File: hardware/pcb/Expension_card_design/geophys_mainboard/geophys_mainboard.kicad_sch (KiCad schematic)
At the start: 0 parts

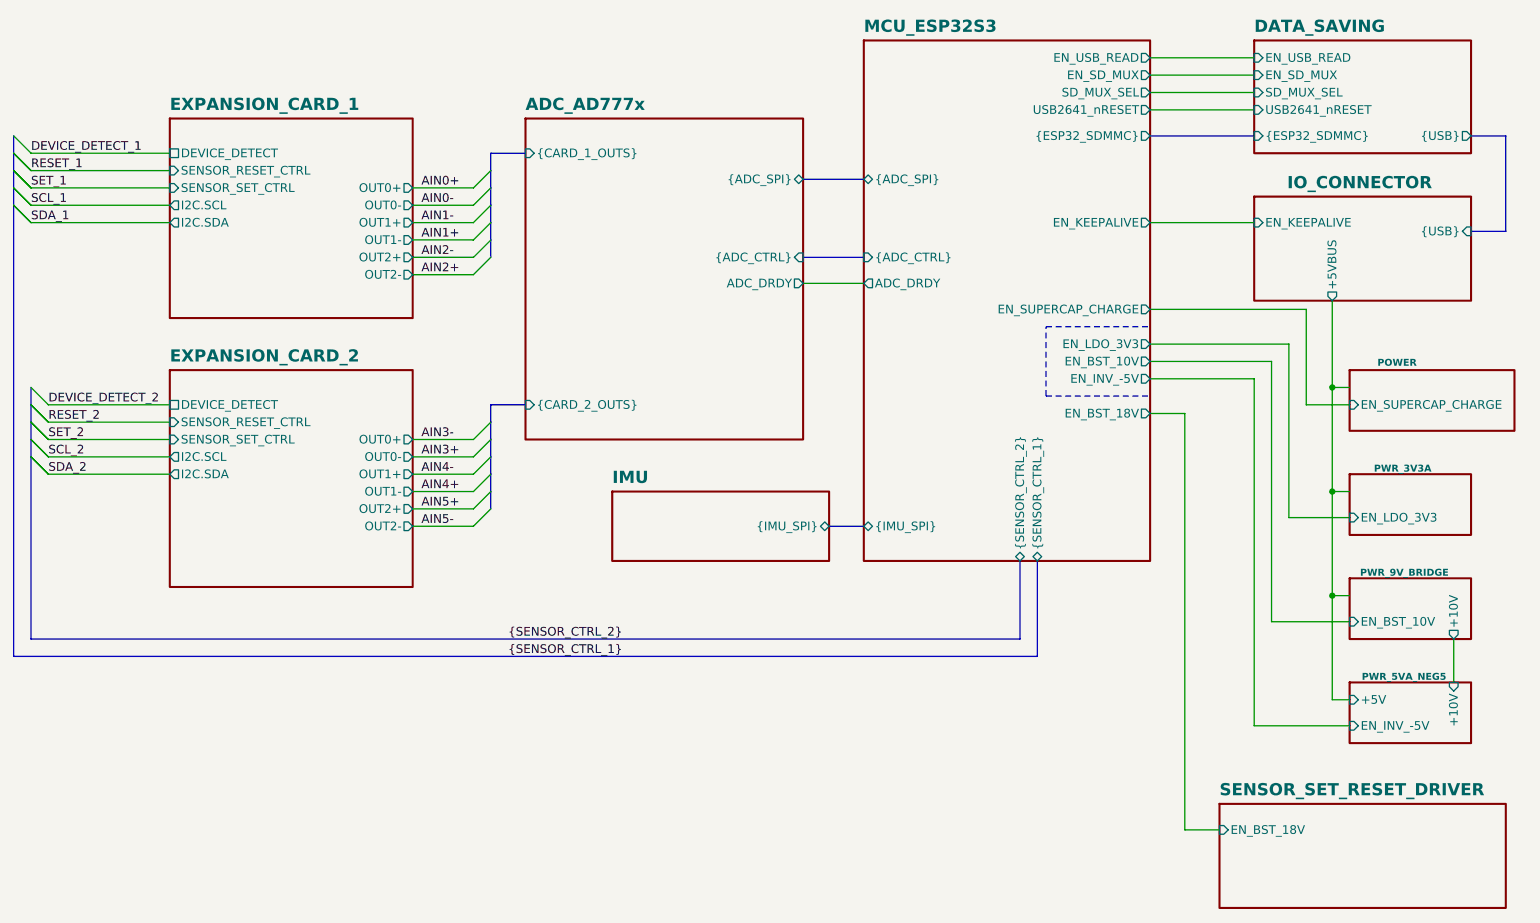
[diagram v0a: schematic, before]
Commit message: ...
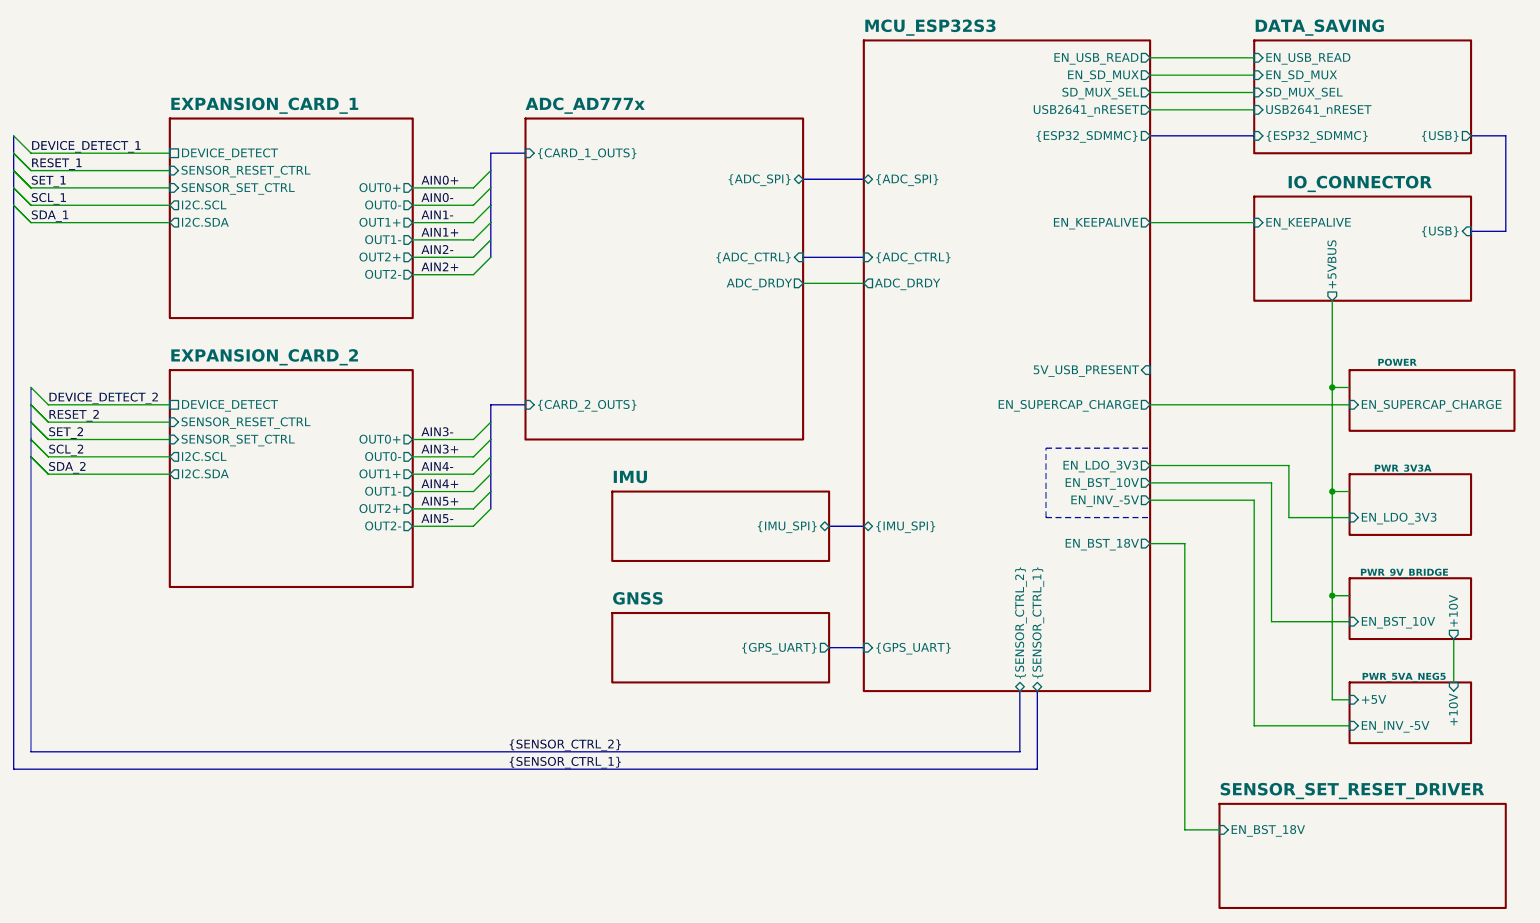
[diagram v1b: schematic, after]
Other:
- added sheet GNSS (schematics/GNSS.kicad_sch)
- sheet MCU_ESP32S3 ports: added 5V_USB_PRESENT, {GPS_UART}; removed none
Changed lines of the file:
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@@
-		)
-	)
-	(bus
-		(pts
-			(xy 176.53 102.87) (xy 176.53 114.3)
-		)
-		(stroke
-			(width 0)
-			(type default)
 		)
 	)
@@
 	(wire
 		(pts
-			(xy 195.58 73.66) (xy 213.36 73.66)
-		)
-		(stroke
-			(width 0)
-			(type default)
-		)
-	)
-	(bus
-		(pts
-			(xy 29.21 116.84) (xy 179.07 116.84)
+			(xy 195.58 91.44) (xy 213.36 91.44)
+		)
+		(stroke
+			(width 0)
+			(type default)
+		)
+	)
+	(bus
+		(pts
+			(xy 29.21 133.35) (xy 179.07 133.35)
 		)
 		(stroke
@@
 	(wire
 		(pts
-			(xy 218.44 80.01) (xy 218.44 66.04)
-		)
-		(stroke
-			(width 0)
-			(type default)
-		)
-	)
-	(wire
-		(pts
 			(xy 87.63 55.88) (xy 96.52 55.88)
 		)
@@
 	(bus
 		(pts
+			(xy 148.59 115.57) (xy 153.67 115.57)
+		)
+		(stroke
+			(width 0)
+			(type default)
+		)
+	)
+	(bus
+		(pts
 			(xy 29.21 48.26) (xy 29.21 50.8)
 		)
@@
 	(bus
 		(pts
+			(xy 176.53 121.92) (xy 176.53 130.81)
+		)
+		(stroke
+			(width 0)
+			(type default)
+		)
+	)
+	(bus
+		(pts
 			(xy 195.58 40.64) (xy 210.82 40.64)
 		)
@@
 	(bus
 		(pts
-			(xy 31.75 114.3) (xy 176.53 114.3)
+			(xy 31.75 130.81) (xy 176.53 130.81)
 		)
 		(stroke
@@
 	(polyline
 		(pts
-			(xy 180.34 78.74) (xy 195.58 78.74)
+			(xy 180.34 96.52) (xy 195.58 96.52)
 		)
 		(stroke
@@
 	(bus
 		(pts
-			(xy 31.75 87.63) (xy 31.75 114.3)
+			(xy 31.75 87.63) (xy 31.75 130.81)
 		)
 		(stroke
@@
 	(wire
 		(pts
-			(xy 210.82 76.2) (xy 210.82 127)
+			(xy 210.82 93.98) (xy 210.82 127)
 		)
 		(stroke
@@
 	(polyline
 		(pts
-			(xy 180.34 68.58) (xy 195.58 68.58)
+			(xy 180.34 86.36) (xy 195.58 86.36)
 		)
 		(stroke
@@
 		)
 	)
+	(bus
+		(pts
+			(xy 179.07 121.92) (xy 179.07 133.35)
+		)
+		(stroke
+			(width 0)
+			(type default)
+		)
+	)
 	(wire
 		(pts
@@
 	(polyline
 		(pts
-			(xy 180.34 78.74) (xy 180.34 68.58)
+			(xy 180.34 96.52) (xy 180.34 86.36)
 		)
 		(stroke
@@
 	(wire
 		(pts
-			(xy 200.66 81.28) (xy 195.58 81.28)
-		)
-		(stroke
-			(width 0)
-			(type default)
-		)
-	)
-	(bus
-		(pts
-			(xy 179.07 102.87) (xy 179.07 116.84)
+			(xy 200.66 100.33) (xy 195.58 100.33)
 		)
 		(stroke
@@
 		)
 	)
-	(wire
-		(pts
-			(xy 224.79 80.01) (xy 218.44 80.01)
-		)
-		(stroke
-			(width 0)
-			(type default)
-		)
-	)
 	(bus
 		(pts
@@
 	(wire
 		(pts
-			(xy 195.58 71.12) (xy 215.9 71.12)
-		)
-		(stroke
-			(width 0)
-			(type default)
-		)
-	)
-	(wire
-		(pts
-			(xy 213.36 73.66) (xy 213.36 111.76)
-		)
-		(stroke
-			(width 0)
-			(type default)
-		)
-	)
-	(wire
-		(pts
-			(xy 200.66 81.28) (xy 200.66 142.24)
+			(xy 195.58 88.9) (xy 215.9 88.9)
+		)
+		(stroke
+			(width 0)
+			(type default)
+		)
+	)
+	(wire
+		(pts
+			(xy 213.36 91.44) (xy 213.36 111.76)
+		)
+		(stroke
+			(width 0)
+			(type default)
+		)
+	)
+	(wire
+		(pts
+			(xy 200.66 100.33) (xy 200.66 142.24)
 		)
 		(stroke
@@
 	(wire
 		(pts
-			(xy 195.58 76.2) (xy 210.82 76.2)
+			(xy 195.58 93.98) (xy 210.82 93.98)
 		)
 		(stroke
@@
 	(wire
 		(pts
-			(xy 195.58 66.04) (xy 218.44 66.04)
+			(xy 195.58 80.01) (xy 224.79 80.01)
 		)
 		(stroke
@@
 	(wire
 		(pts
-			(xy 215.9 71.12) (xy 215.9 96.52)
+			(xy 215.9 88.9) (xy 215.9 96.52)
 		)
 		(stroke
@@
 	(bus
 		(pts
-			(xy 29.21 50.8) (xy 29.21 116.84)
+			(xy 29.21 50.8) (xy 29.21 133.35)
 		)
 		(stroke
@@
 	)
 	(label "{SENSOR_CTRL_2}"
-		(at 101.6 114.3 0)
+		(at 101.6 130.81 0)
 		(effects
 			(font
@@
 	)
 	(label "{SENSOR_CTRL_1}"
-		(at 101.6 116.84 0)
+		(at 101.6 133.35 0)
 		(effects
 			(font
@@
 	(sheet
 		(at 153.67 26.67)
-		(size 41.91 76.2)
+		(size 41.91 95.25)
 		(exclude_from_sim no)
 		(in_bom yes)
@@
 		)
 		(property "Sheetfile" "schematics/mcu_esp32s3.kicad_sch"
-			(at 153.67 103.5308 0)
+			(at 153.67 122.5808 0)
 			(effects
 				(font
@@
 		)
 		(pin "EN_INV_-5V" output
-			(at 195.58 76.2 0)
+			(at 195.58 93.98 0)
 			(effects
 				(font
@@
 		)
 		(pin "EN_LDO_3V3" output
-			(at 195.58 71.12 0)
+			(at 195.58 88.9 0)
 			(effects
 				(font
@@
 		)
 		(pin "EN_BST_10V" output
-			(at 195.58 73.66 0)
+			(at 195.58 91.44 0)
 			(effects
 				(font
@@
 		)
 		(pin "EN_BST_18V" output
-			(at 195.58 81.28 0)
+			(at 195.58 100.33 0)
 			(effects
 				(font
@@
 		)
 		(pin "EN_SUPERCAP_CHARGE" output
-			(at 195.58 66.04 0)
+			(at 195.58 80.01 0)
 			(effects
 				(font
@@
 		)
 		(pin "{SENSOR_CTRL_1}" bidirectional
-			(at 179.07 102.87 270)
+			(at 179.07 121.92 270)
 			(effects
 				(font
@@
 		)
 		(pin "{SENSOR_CTRL_2}" bidirectional
-			(at 176.53 102.87 270)
+			(at 176.53 121.92 270)
+			(effects
+				(font
+					(size 1.27 1.27)
+				)
+				(justify left)
+			)
+		)
+		(pin "5V_USB_PRESENT" input
+			(at 195.58 74.93 0)
+			(effects
+				(font
+					(size 1.27 1.27)
+				)
+				(justify right)
+			)
+		)
+		(pin "{GPS_UART}" input
+			(at 153.67 115.57 180)
 			(effects
 				(font
@@
 				)
 			)
+		)
+	)
+	(sheet
+		(at 116.84 110.49)
+		(size 31.75 10.16)
+		(exclude_from_sim no)
+		(in_bom yes)
+		(on_board yes)
+		(dnp no)
+		(fields_autoplaced yes)
+		(stroke
+			(width 0.3048)
+			(type solid)
+			(color 0 0 0 1)
+		)
+		(fill
+			(color 194 194 194 0.4200)
+		)
+		(property "Sheetname" "GNSS"
+			(at 116.84 109.4482 0)
+			(effects
+				(font
+					(size 1.778 1.778)
+					(thickness 0.4064)
+					(bold yes)
+					(color 0 0 0 1)
+				)
+				(justify left bottom)
+			)
+		)
+		(property "Sheetfile" "schematics/GNSS.kicad_sch"
+			(at 116.84 121.3108 0)
+			(effects
+				(font
+					(size 1.27 1.27)
+				)
+				(justify left top)
+				(hide yes)
+			)
+		)
+		(pin "{GPS_UART}" output
+			(at 148.59 115.57 0)
+			(effects
+				(font
+					(size 1.27 1.27)
+				)
+				(justify right)
+			)
+		)
+		(instances
+			(project "geophys_mainboard"
+				(path "/b5f9ef85-43f0-43d8-a1fd-ed489b1654c1"
+					(page "14")
+				)
+			)
